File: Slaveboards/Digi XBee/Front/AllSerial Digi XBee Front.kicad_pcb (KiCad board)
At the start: 2 copper layers, 71.5 x 24 mm, 3 parts

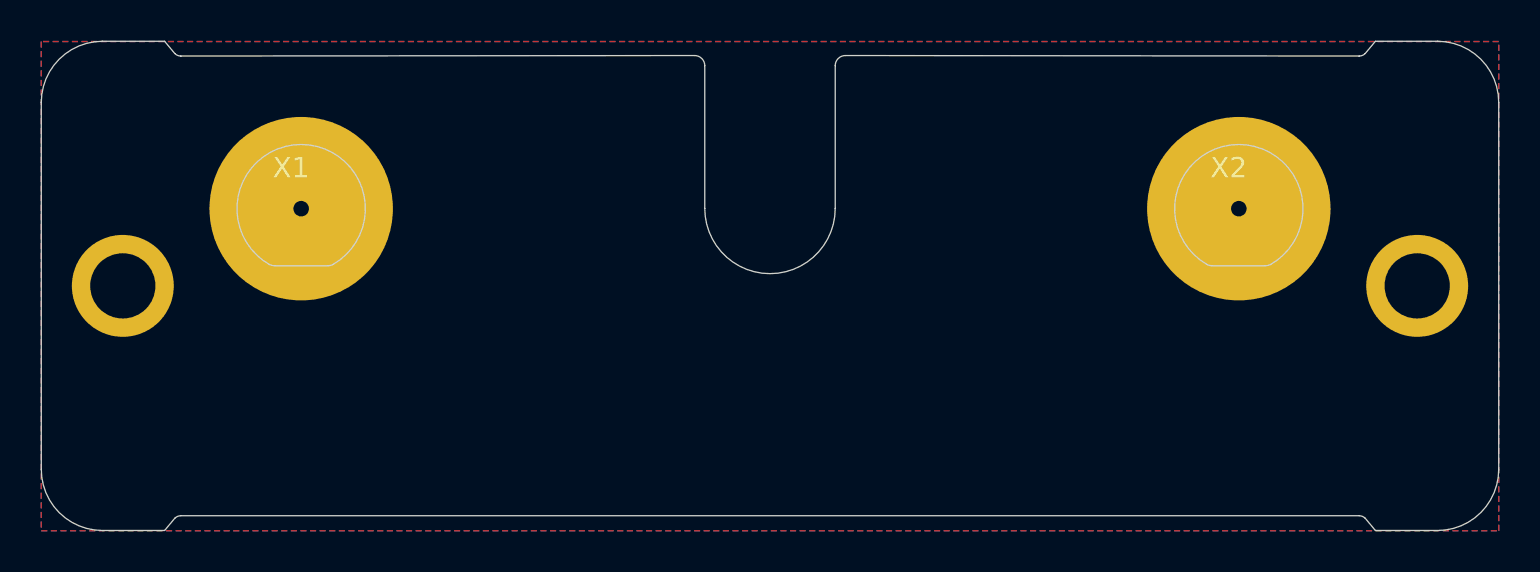
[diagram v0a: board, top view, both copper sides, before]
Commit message: Improve libraries
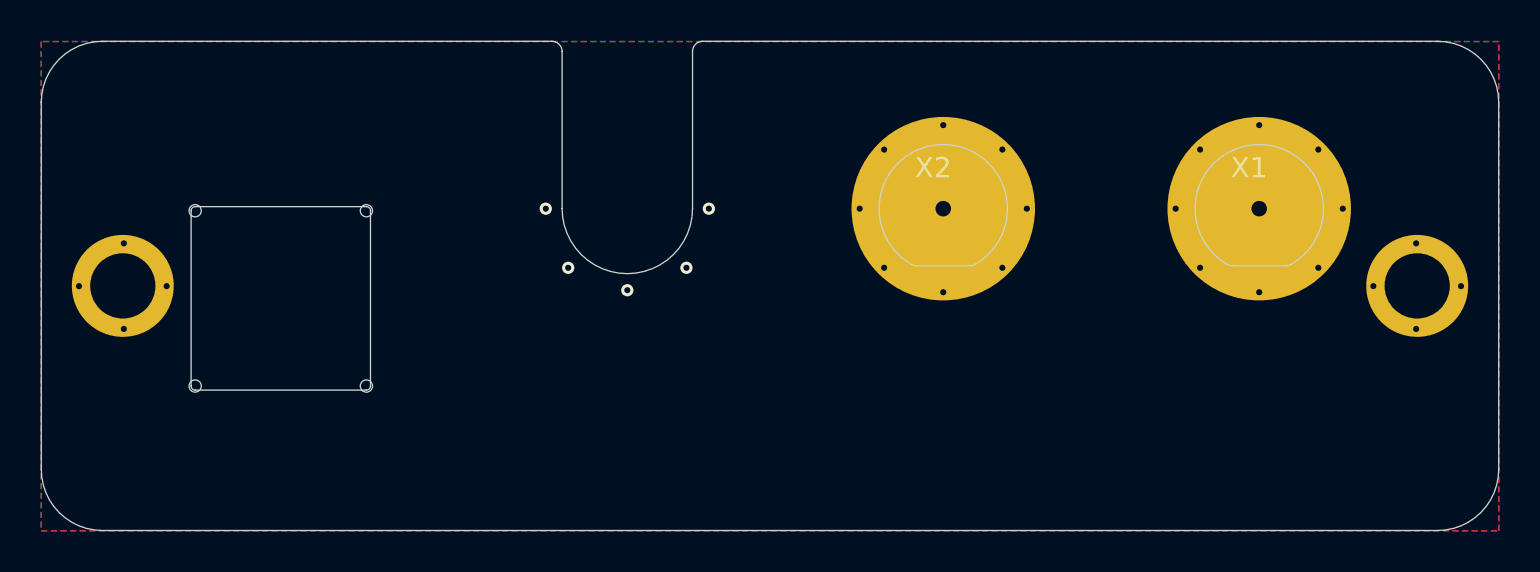
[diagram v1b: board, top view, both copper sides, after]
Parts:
- added REF**: Val**, AllSerial:Metz_PT11302HBBN_182, F.Cu at (121.7, 102.0)
- moved X1 47.0 mm to (169.7, 86.2)
- moved X2 14.5 mm to (154.2, 86.2)
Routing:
- net GND: vias 0 -> 29
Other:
- outline, holes or cut-outs redrawn
- board text added: "All Serial Digi XBee Front v1.0 27/25"
- board text added: "Digi XBee"
- board text added: "JLCJLCJLCJLC"
